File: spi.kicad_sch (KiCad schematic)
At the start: 24 parts, among them CN2 CAN, CN5 THERMO1, CN6 THERMO2, CN7 CAN, IC2 MAX31855K, IC3 MAX31855K, IC4 MCP2515-xSO, IC5 TCAN332DR, IC6 LSM6DSOTR, J3 CAN_TERM, T6 TEST_CAN, Y1 8MHz

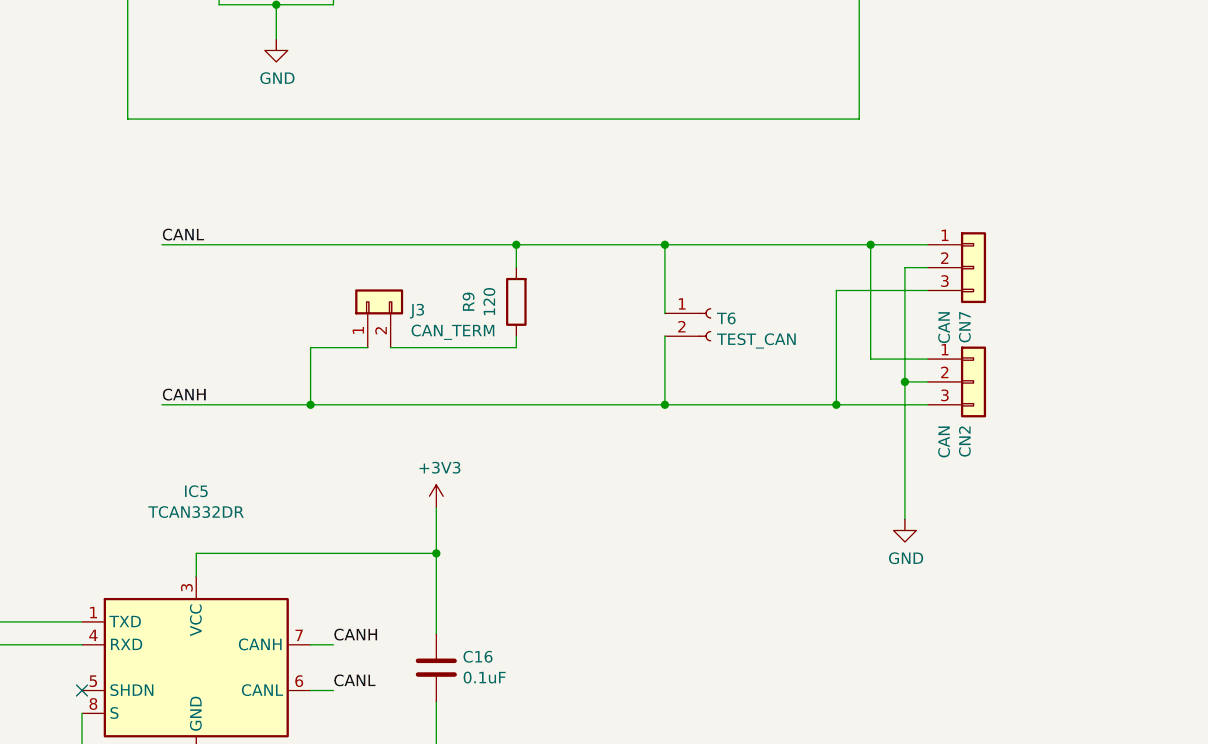
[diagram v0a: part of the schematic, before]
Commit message: hello
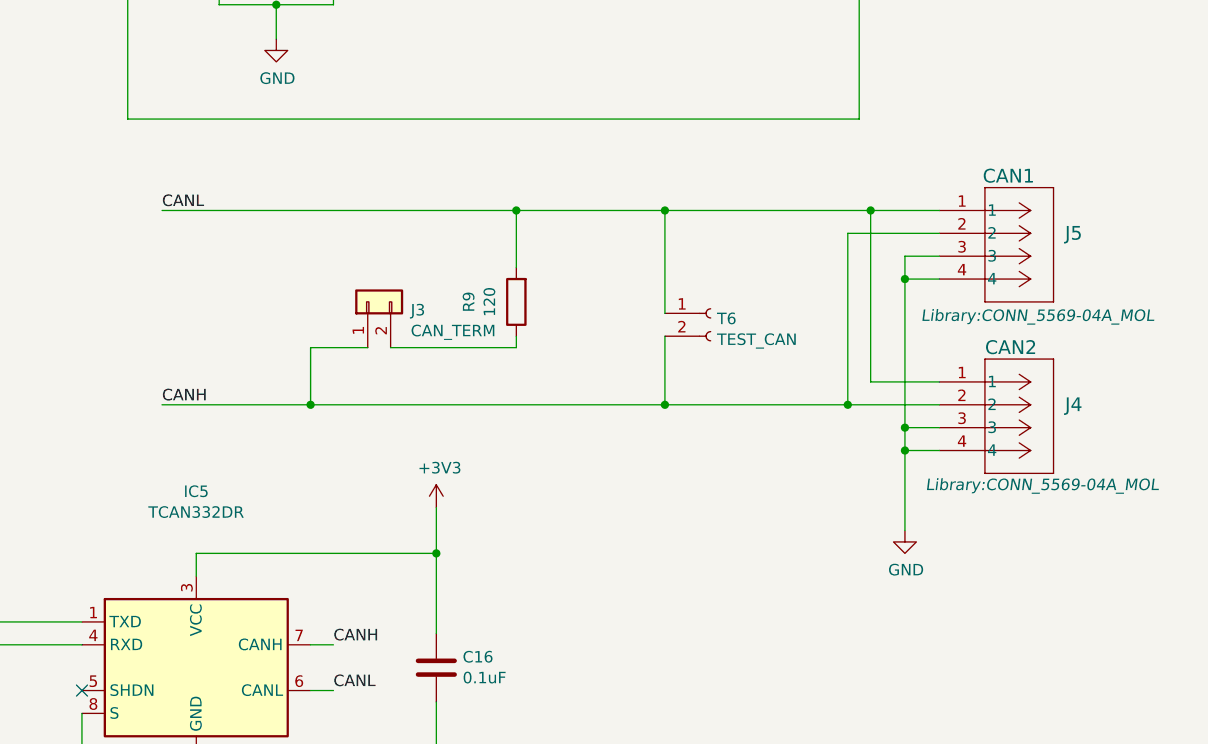
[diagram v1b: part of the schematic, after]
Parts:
- removed CN2, CN7: CAN, telemetry-pcb:molex-sl-1x03-horizontal, symbol Connector_Generic:Conn_01x03
- added J4: CAN2, Library:CONN_5569-04A_MOL, symbol 2025-11-01_18-29-52:39301040
- added J5: CAN1, Library:CONN_5569-04A_MOL, symbol 2025-11-01_18-29-52:39301040
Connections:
- net CANH: now also J4.2, J5.2
- net CANL: now also J4.1, J5.1
- net GND: now also J4.3, J4.4, J5.3, J5.4
